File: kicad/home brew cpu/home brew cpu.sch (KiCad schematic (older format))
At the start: 18 parts

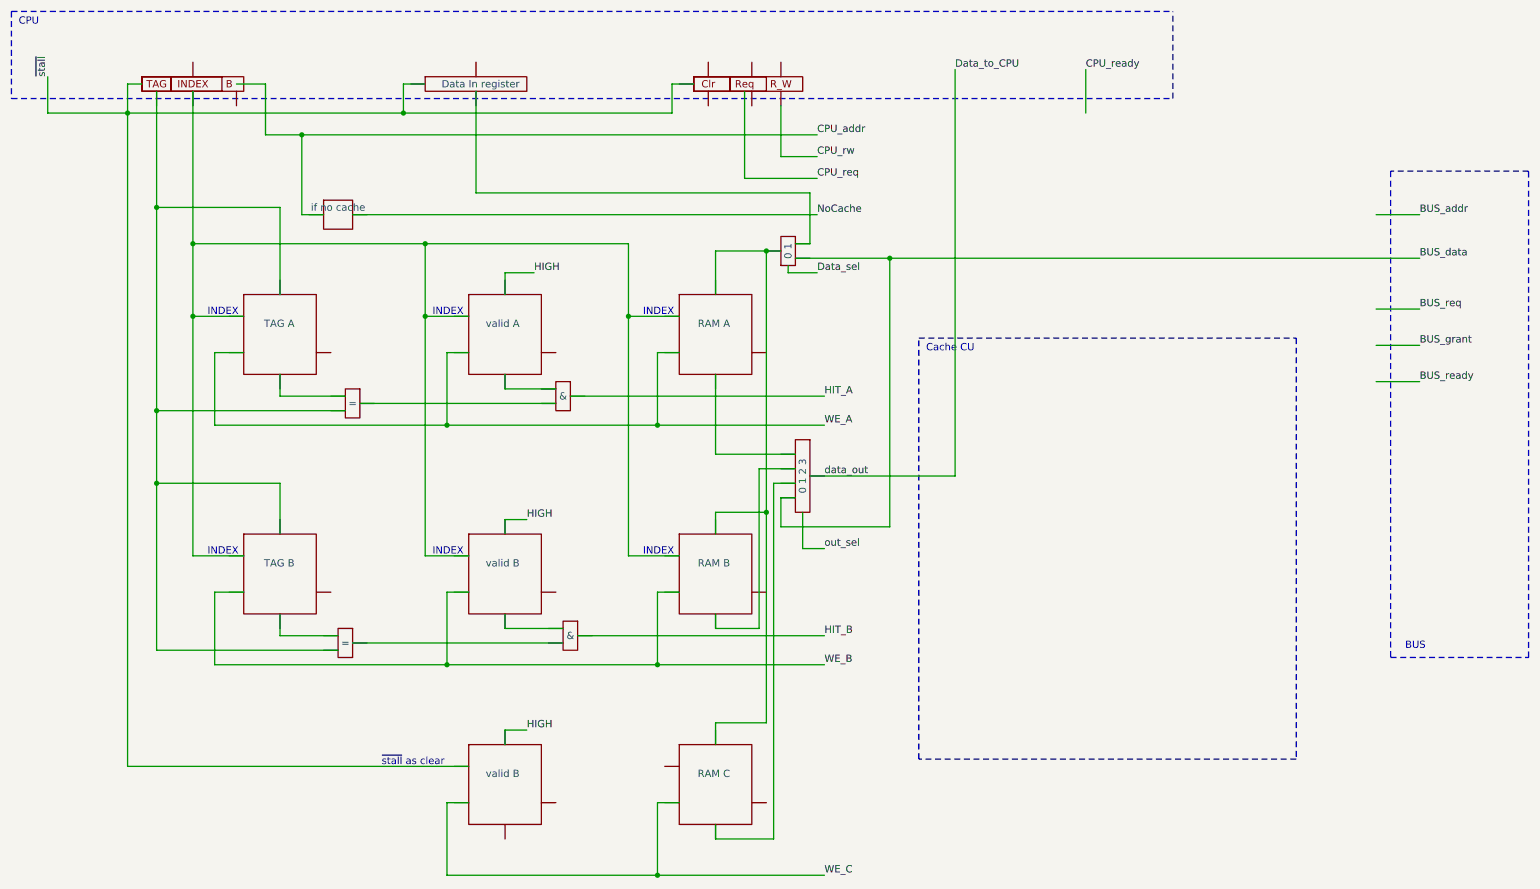
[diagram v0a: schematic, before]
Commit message: clean the git repo
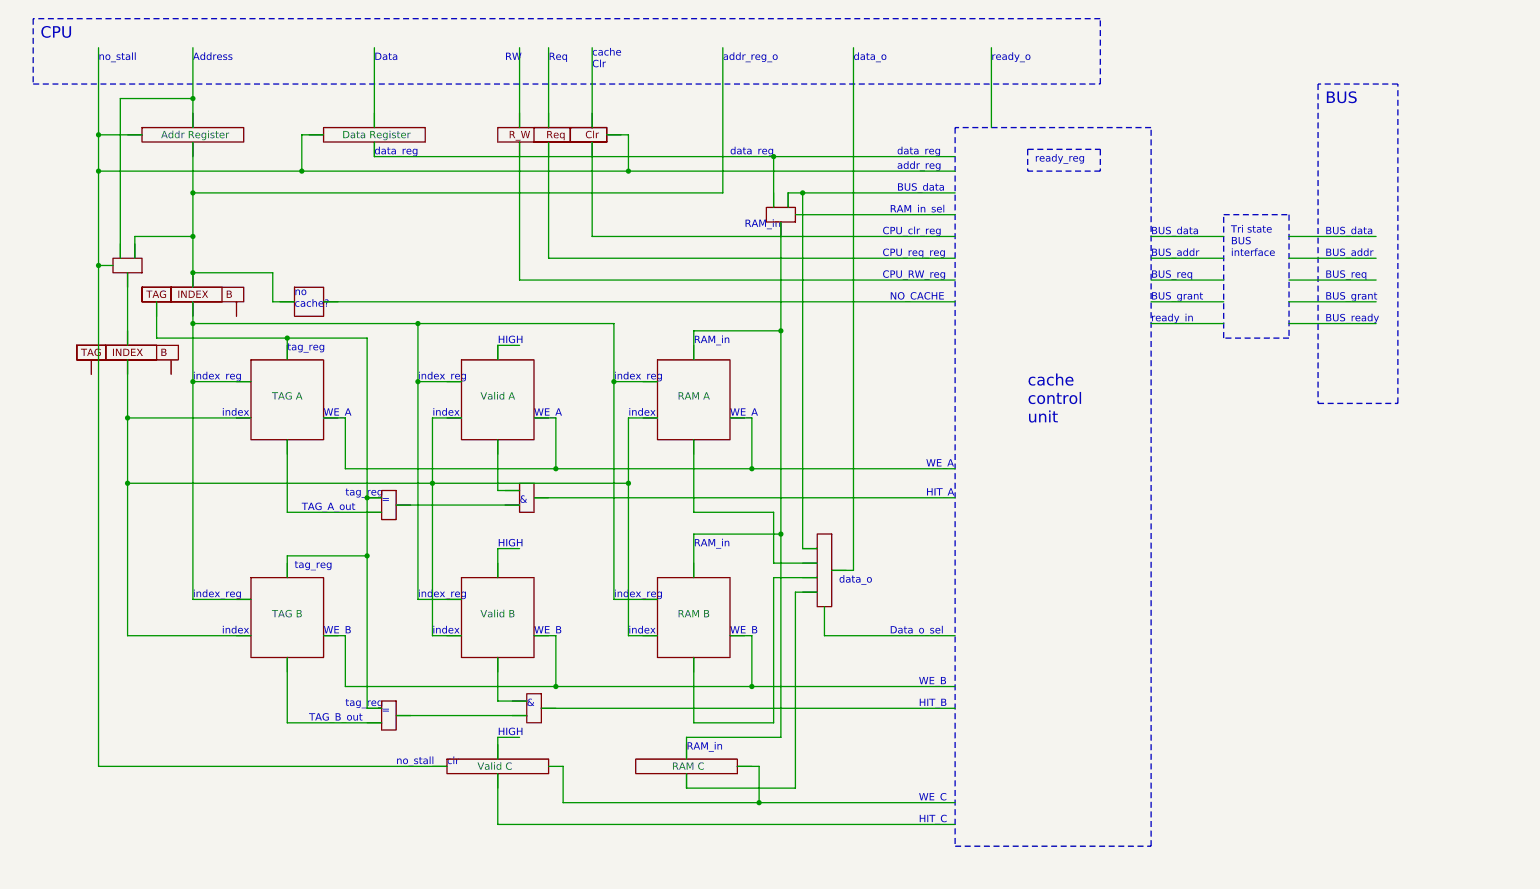
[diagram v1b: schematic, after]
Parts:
- removed U?: Data In register, symbol New_Library:register
- removed U?: PCregister, symbol New_Library:PCregister
- removed U?: controlreg, symbol New_Library:controlreg
- removed U?: TAG A, symbol New_Library:RAM
- removed U?: valid A, symbol New_Library:RAM
- removed U?: RAM A, symbol New_Library:RAM
- removed U?: TAG B, symbol New_Library:RAM
- removed U? (x2): valid B, symbol New_Library:RAM
- removed U?: RAM B, symbol New_Library:RAM
- removed U?: RAM C, symbol New_Library:RAM
- removed U? (x2): =, symbol 4xxx:2-1
- removed U? (x2): &, symbol 4xxx:2-1
- removed U?: if no cache, symbol New_Library:1to1
- removed U?: 0 1, symbol 4xxx:2-1
- removed U?: 0 1 2 3, symbol New_Library:4to1
- added U?: TAG A, symbol New_Library:RAM
- added U?: TAG B, symbol New_Library:RAM
- added U?: Valid A, symbol New_Library:RAM
- added U?: Valid B, symbol New_Library:RAM
- added U?: Valid C, symbol New_Library:register
- added U?: RAM A, symbol New_Library:RAM
- added U?: RAM B, symbol New_Library:RAM
- added U?: RAM C, symbol New_Library:register
- added U?: Addr Register, symbol New_Library:register
- added U?: Data Register, symbol New_Library:register
- added U? (x2): PCregister, symbol New_Library:PCregister
- added U? (x6): 2-1, symbol 4xxx:2-1
- added U?: no cache, symbol New_Library:1to1
- added U?: 4to1, symbol New_Library:4to1
- added ds: controlreg, symbol New_Library:controlreg
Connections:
- net labels removed: BUS_addr, BUS_data, BUS_grant, BUS_ready, BUS_req, CPU_addr, CPU_ready, CPU_req, CPU_rw, Data_sel, Data_to_CPU, HIGH, HIT_A, HIT_B, NoCache, WE_A, WE_B, WE_C, data_out, out_sel, ~stall
- wire segments 130 -> 172
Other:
- note added: "&"
- note added: "="
- note added: "Address"
- note added: "BUS_addr"
- note added: "BUS_data"
- note added: "BUS_grant"
- note added: "BUS_ready"
- note added: "BUS_req"
- note added: "CPU_RW_reg"
- note added: "CPU_clr_reg"
- note added: "CPU_req_reg"
- note added: "Data"
- note added: "Data_o_sel"
- note added: "HIGH"
- note added: "HIT_A"
- note added: "HIT_B"
- note added: "HIT_C"
- note added: "NO_CACHE"
- note added: "RAM_in"
- note added: "RAM_in_sel"
- note added: "RW"
- note added: "Req"
- note added: "TAG_A_out"
- note added: "TAG_B_out"
- note added: "Tri state\nBUS \ninterface"
- note added: "WE_A"
- note added: "WE_B"
- note added: "WE_C"
- note added: "addr_reg"
- note added: "addr_reg_o"
- note added: "cache\nClr"
- note added: "cache\ncontrol\nunit"
- note added: "clr"
- note added: "data_o"
- note added: "data_reg"
- note added: "index"
- note added: "index_reg"
- note added: "no \ncache?"
- note added: "no_stall"
- note added: "ready_in"
- note added: "ready_o"
- note added: "ready_reg"
- note added: "tag_reg"
- note removed: "Cache CU"
- note removed: "INDEX"
- note removed: "~stall as clear"
